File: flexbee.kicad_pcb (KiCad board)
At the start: 4 copper layers, 30.7 x 17.6 mm, 68 parts, among them J1 Conn_01x12_Male, J2 Conn_01x12_Male, U1 SSD210, U2 ea3056, U3 spinor, Y1 Crystal_GND24

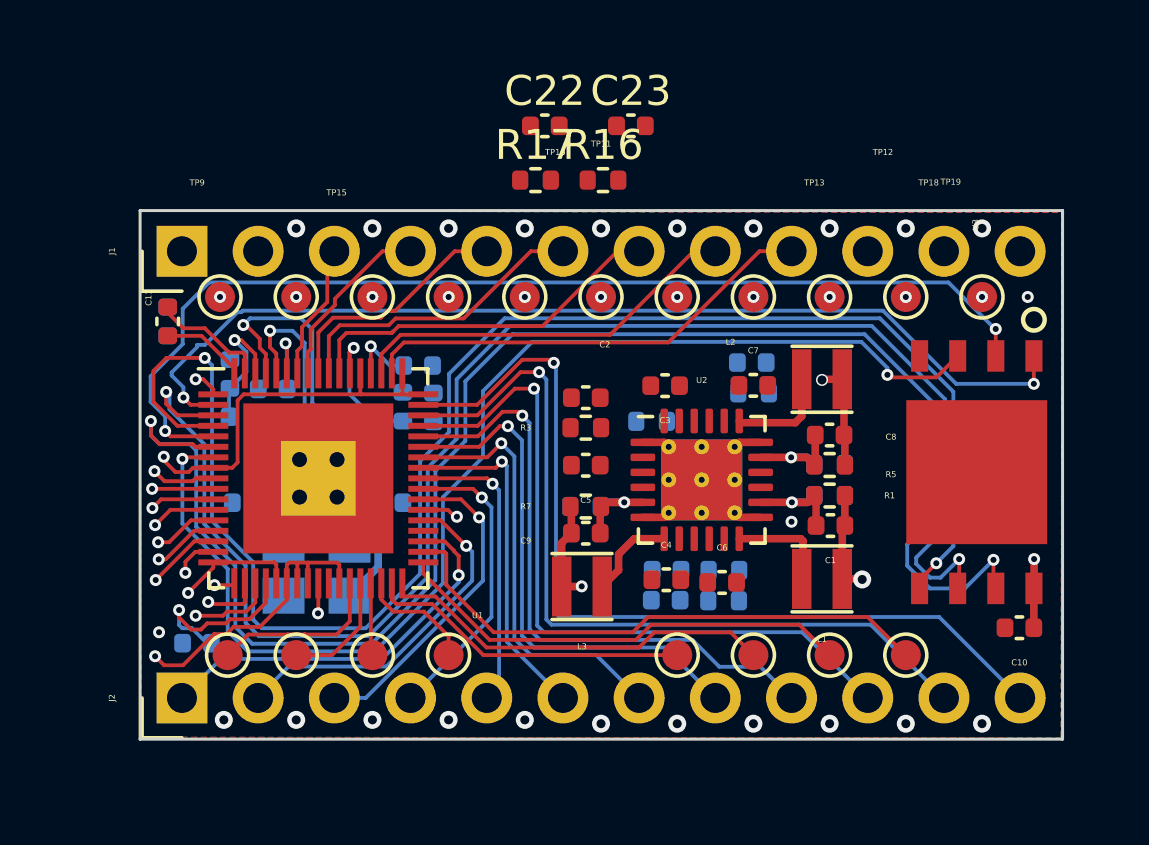
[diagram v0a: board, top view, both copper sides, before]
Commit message: Layout work.
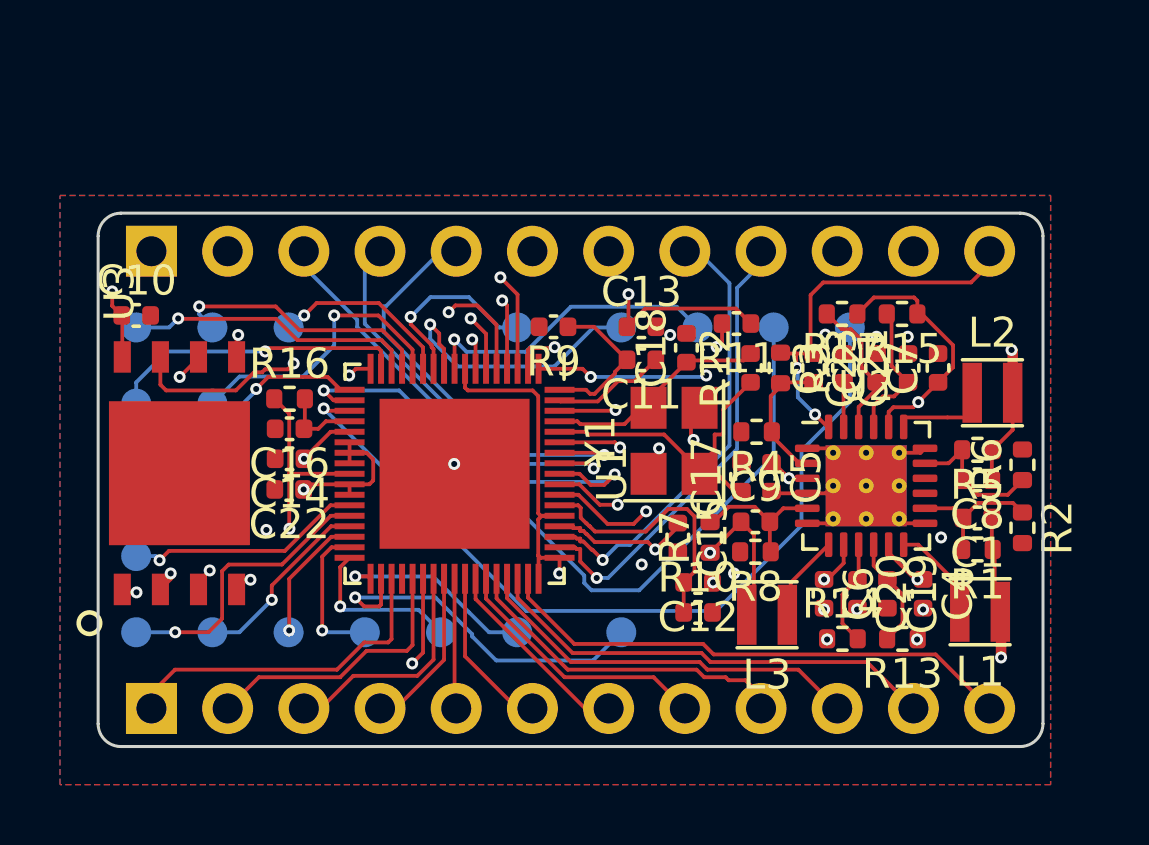
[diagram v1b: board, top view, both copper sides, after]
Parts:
- C12, C13, C14, C15, C16, C17, C18, C19, C20, C21, R10, R11, R12, R13, R14, R15, R2, R4, R6, R8, R9, Y1: moved to F.Cu
- J1, J2, TP1, TP10, TP11, TP12, TP13, TP14, TP15, TP16, TP17, TP18, TP19, TP2, TP3, TP4, TP5, TP6, TP7, TP8, TP9: moved to B.Cu
- moved C10 31.2 mm to (127.0, 88.5), turned to 0 degrees
- moved U3 26.6 mm to (128.4, 93.8), turned to 90 degrees
- moved TP13 23.9 mm to (127.0, 94.0)
- moved TP18 20.9 mm to (127.0, 91.4)
- moved TP12 18.1 mm to (127.0, 88.9)
- moved R11 16.7 mm to (147.0, 88.8), turned to 180 degrees
- moved C17 16.5 mm to (147.2, 93.9), turned to 90 degrees
- moved TP9 15.9 mm to (145.7, 88.9)
- moved C11 15.8 mm to (143.8, 90.0), turned to 180 degrees
- moved C22 14.8 mm to (132.1, 94.3), turned to 180 degrees
- moved R12 14.5 mm to (147.5, 90.2), turned to 90 degrees
- moved C13 13.8 mm to (143.8, 88.9), turned to 0 degrees
- moved TP17 13.0 mm to (129.5, 88.9)
- moved R9 12.9 mm to (140.9, 88.9), turned to 180 degrees
- moved R16 12.7 mm to (132.1, 91.3)
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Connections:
- J1 pad 3: /sar_gpio0 -> /sar_gpio2
- J1 pad 5: /sar_gpio2 -> /sar_gpio0
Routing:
- net /flash_mosi: track 53.7 -> 12.6 mm
- net /flash_hld: track 53.7 -> 14.2 mm
- net /flash_clk: track 51.7 -> 16.3 mm
- net +3V3: track 67.5 -> 41.1 mm, vias 6 -> 9
- net /flash_wpz: track 40.2 -> 15.1 mm
- net Net-(TP13-Pad1): track 26.4 -> 8.74 mm, vias 2 -> 1
- net Net-(TP18-Pad1): track 25.4 -> 9.98 mm, vias 2 -> 1
- net Net-(TP12-Pad1): track 25.0 -> 9.70 mm, vias 2 -> 1
- net /flash_miso: track 35.4 -> 20.2 mm
- net /lineout: track 26.9 -> 11.8 mm, vias 1 -> 2
- net Net-(TP17-Pad1): track 21.8 -> 8.87 mm, vias 2 -> 1
- net VBUS: track 0.00 -> 12.9 mm, vias 0 -> 2
- net VCC: track 0.00 -> 12.7 mm, vias 0 -> 6
- net /ttl21: track 30.0 -> 17.5 mm, vias 1 -> 0
- net /ttl20: track 27.1 -> 15.4 mm, vias 1 -> 0
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- added copper zone on In2.Cu, net +3V3
- added copper zone on In2.Cu, net VCC
- removed copper zone on In2.Cu, net GND
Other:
- board size 30.7 x 17.6 mm -> 31.5 x 17.8 mm
